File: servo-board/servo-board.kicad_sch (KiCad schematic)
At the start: 9 parts, among them J1 Screw_Terminal_01x02, J2 Screw_Terminal_01x02, J3 Conn_02x10_Counter_Clockwise, U1 ESP32-S3-DEVKITC-1-N8R8, U2 GY-521_MPU-6050

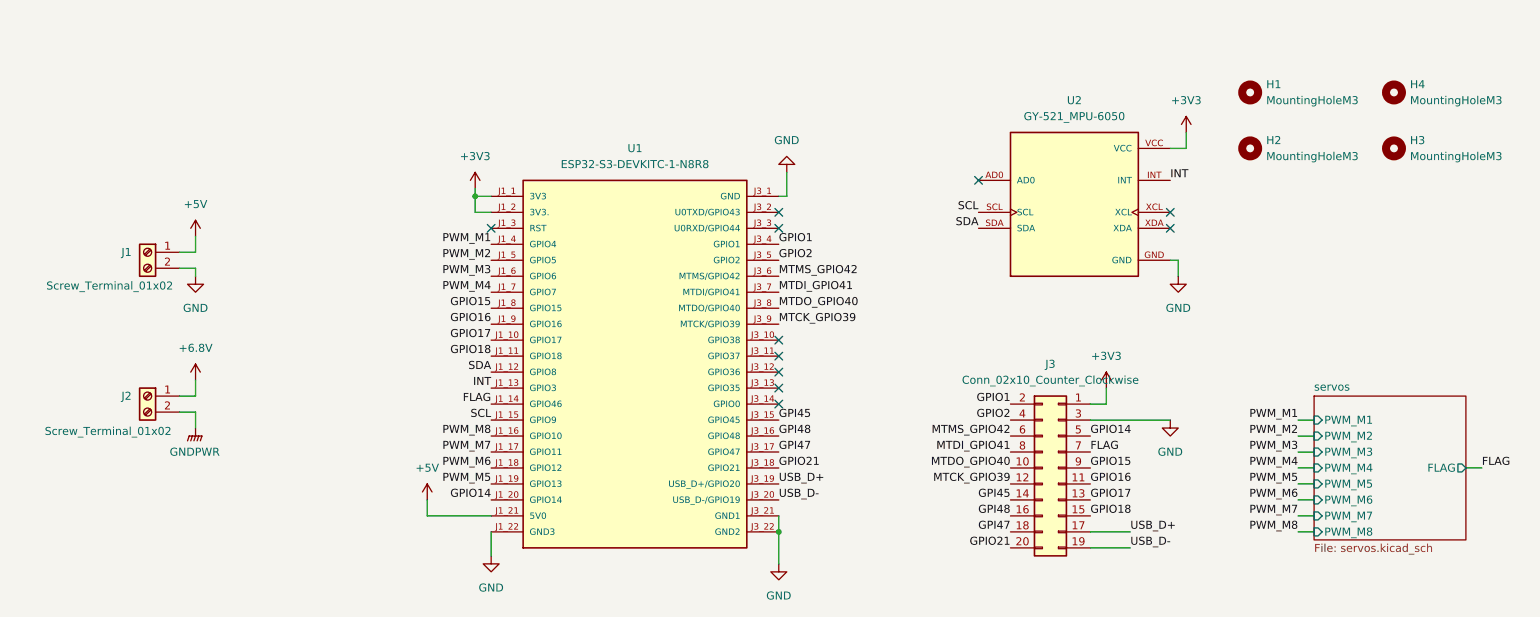
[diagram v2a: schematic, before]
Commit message: changes
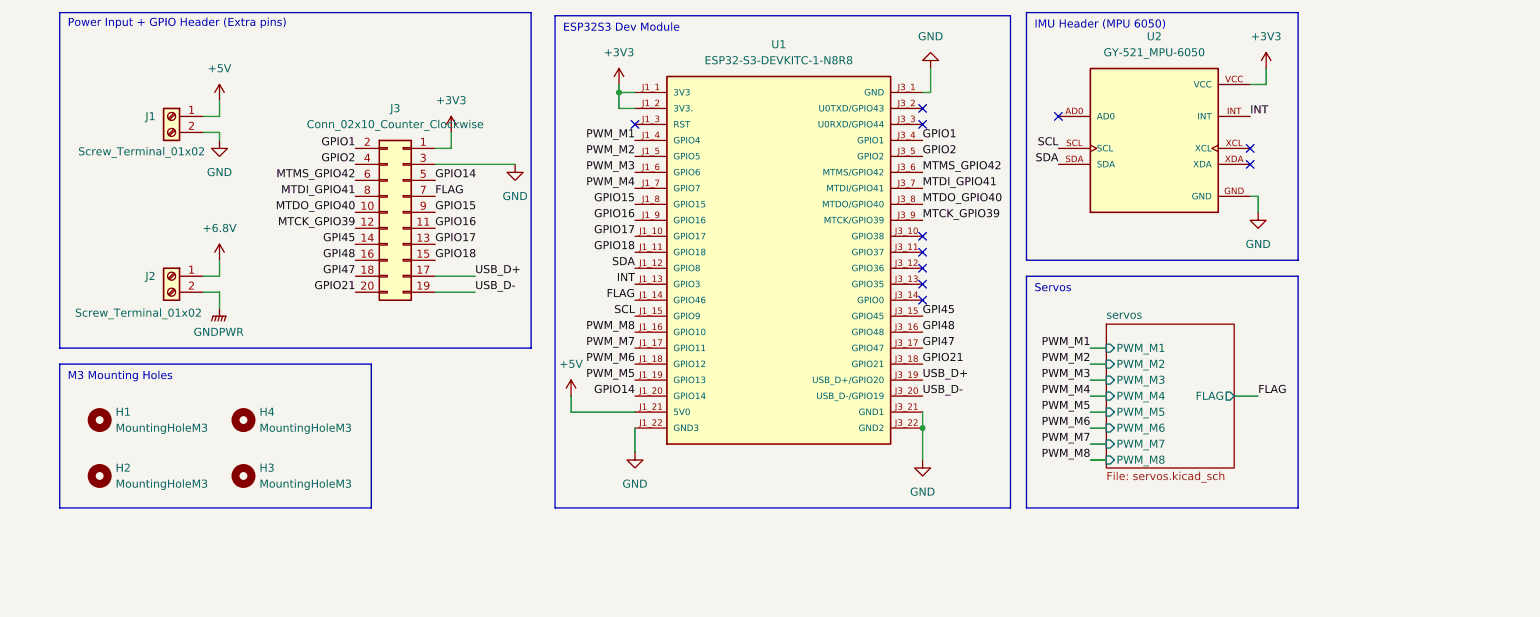
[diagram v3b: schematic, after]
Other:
- note added: "ESP32S3 Dev Module"
- note added: "IMU Header (MPU 6050)"
- note added: "M3 Mounting Holes"
- note added: "Power Input + GPIO Header (Extra pins)"
- note added: "Servos"
- moved on the sheet: H1, H2, H3, H4, J1, J2, J3, U1, U2
